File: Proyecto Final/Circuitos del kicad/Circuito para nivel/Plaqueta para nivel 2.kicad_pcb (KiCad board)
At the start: 2 copper layers, 60 x 44 mm, 20 parts, among them J1 Conn_01x05, J2 Conn_01x03, Q1 BC557, Q2 BC557, Q3 BC557, Q4 BC557, U1 ULN2003A

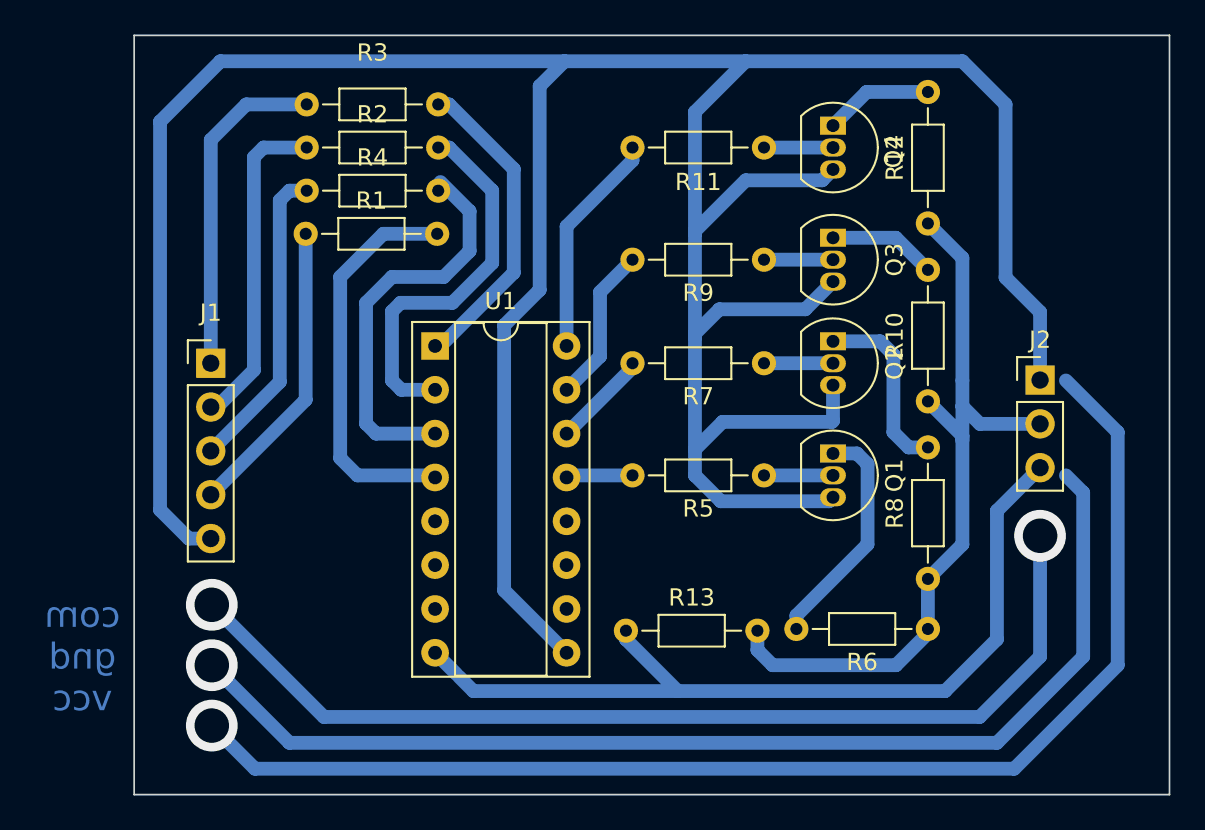
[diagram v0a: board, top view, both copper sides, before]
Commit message: Placas bien subidas
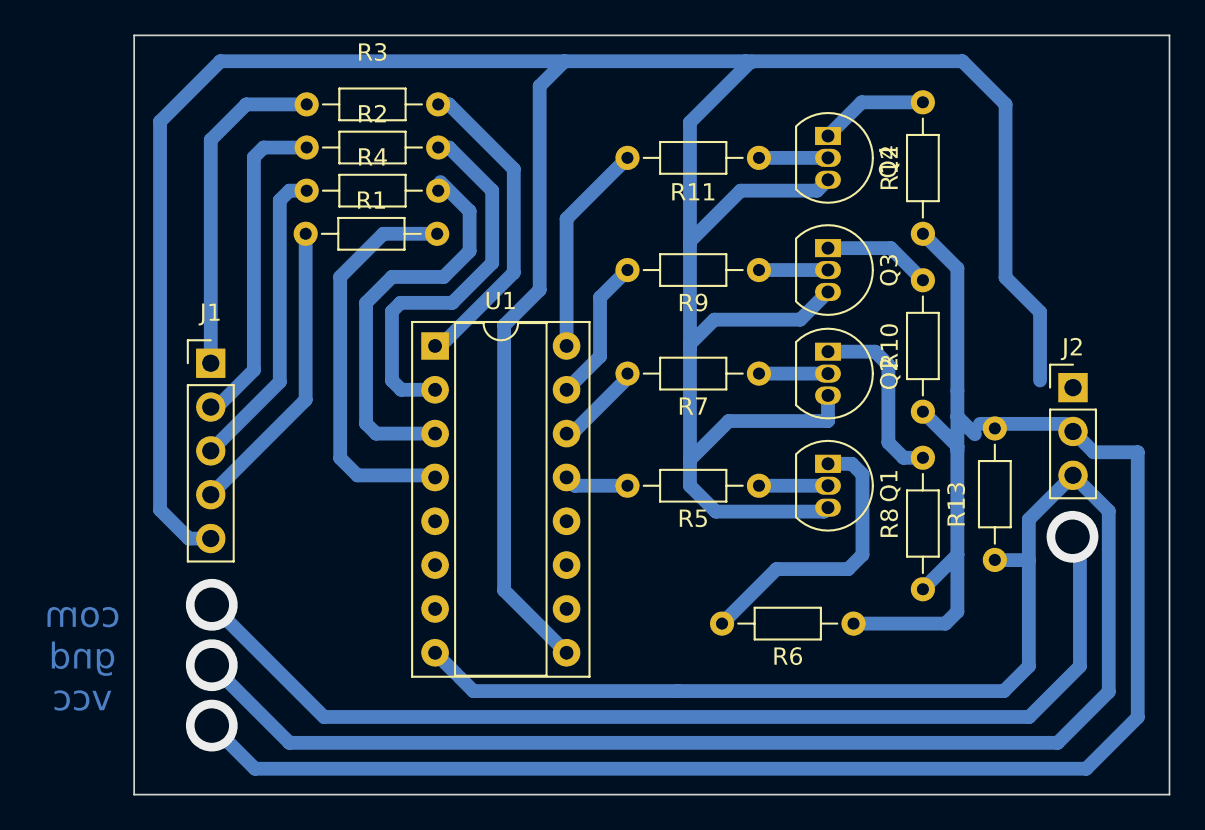
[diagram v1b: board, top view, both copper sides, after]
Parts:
- moved R13 21.8 mm to (158.9, 116.9), turned to 90 degrees
- moved R6 4.32 mm to (150.7, 120.6)
- moved J2 1.96 mm to (163.4, 106.9)
- moved R10 0.67 mm to (154.7, 108.3)
- moved Q1 0.67 mm to (149.2, 111.3)
- moved Q2 0.67 mm to (149.2, 104.8)
- moved Q3 0.67 mm to (149.2, 98.8)
- moved Q4 0.67 mm to (149.2, 92.3)
- moved R11 0.67 mm to (145.2, 93.6)
- moved R12 0.67 mm to (154.7, 98.0)
- moved R5 0.67 mm to (145.2, 112.6)
- moved R7 0.67 mm to (145.2, 106.1)
- moved R8 0.67 mm to (154.7, 118.6)
- moved R9 0.67 mm to (145.2, 100.1)
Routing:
- net GND: track 96.0 -> 297.9 mm
- net (no net): track 198.3 -> 0.00 mm
- net Net-(Q1-Pad1): track 13.5 -> 16.7 mm
- net Net-(R9-Pad2): track 9.12 -> 8.40 mm
- net Net-(R11-Pad2): track 13.1 -> 12.4 mm
- net +5V: track 195.5 -> 196.1 mm
- net Net-(R7-Pad2): track 5.66 -> 5.12 mm

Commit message: jhjkhn
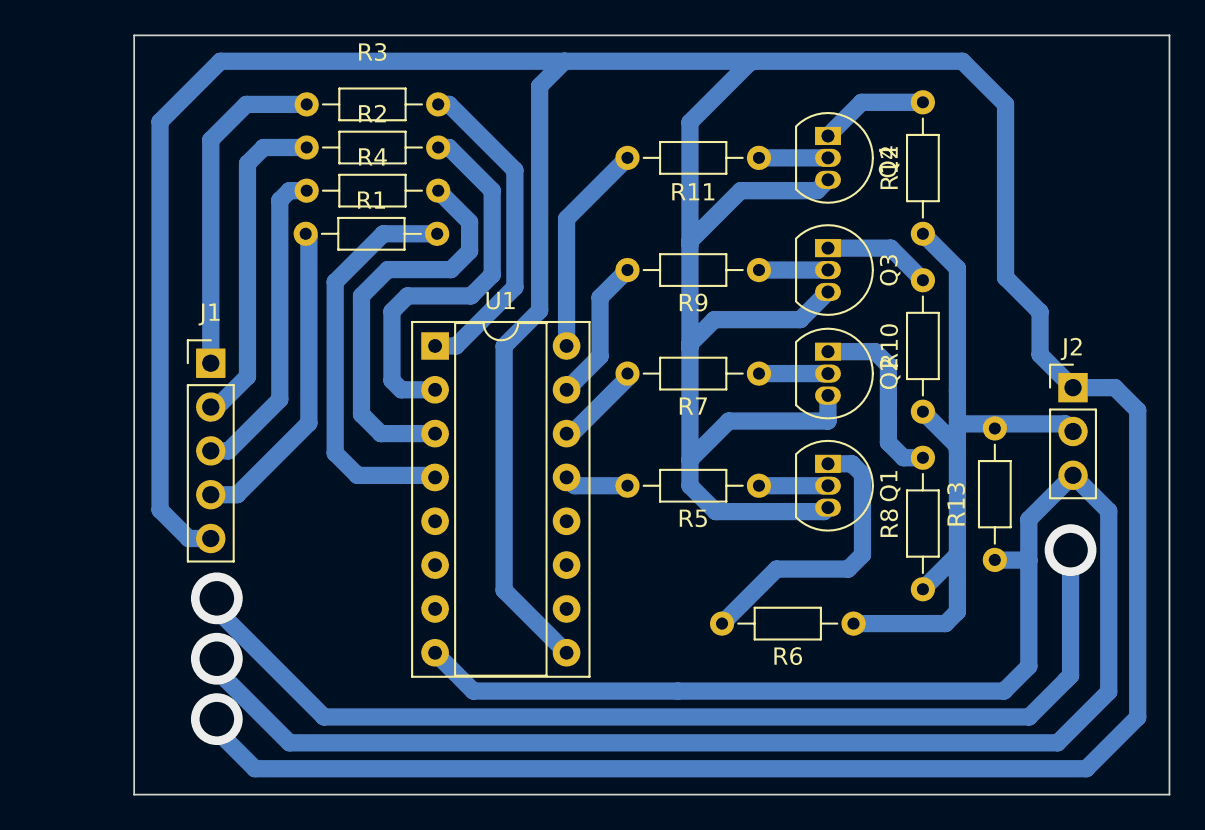
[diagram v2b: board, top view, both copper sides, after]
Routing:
- net +5V: track 196.1 -> 275.3 mm, vias 0 -> 1
- net GND: track 297.9 -> 221.1 mm, vias 0 -> 1
- net Net-(J1-Pad4): track 17.4 -> 18.4 mm
- net Net-(J1-Pad3): track 18.0 -> 18.6 mm
- net Net-(R3-Pad2): track 18.3 -> 18.8 mm
- net (no net): vias 4 -> 2
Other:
- board text removed: "com gnd vcc"

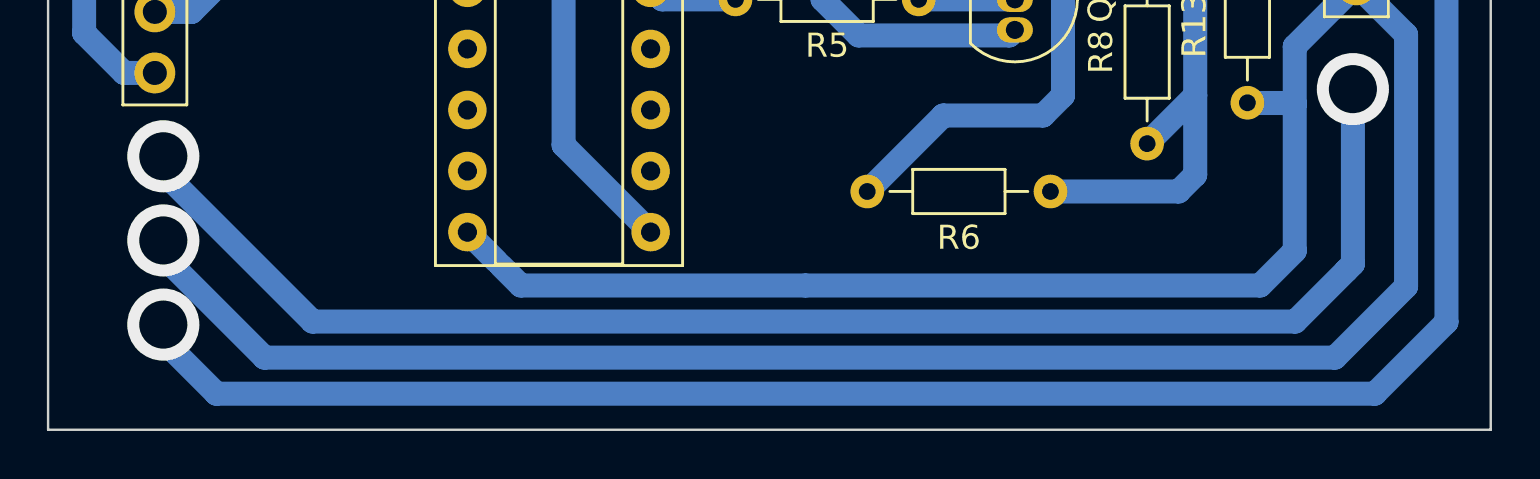
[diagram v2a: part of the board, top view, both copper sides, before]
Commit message: |a
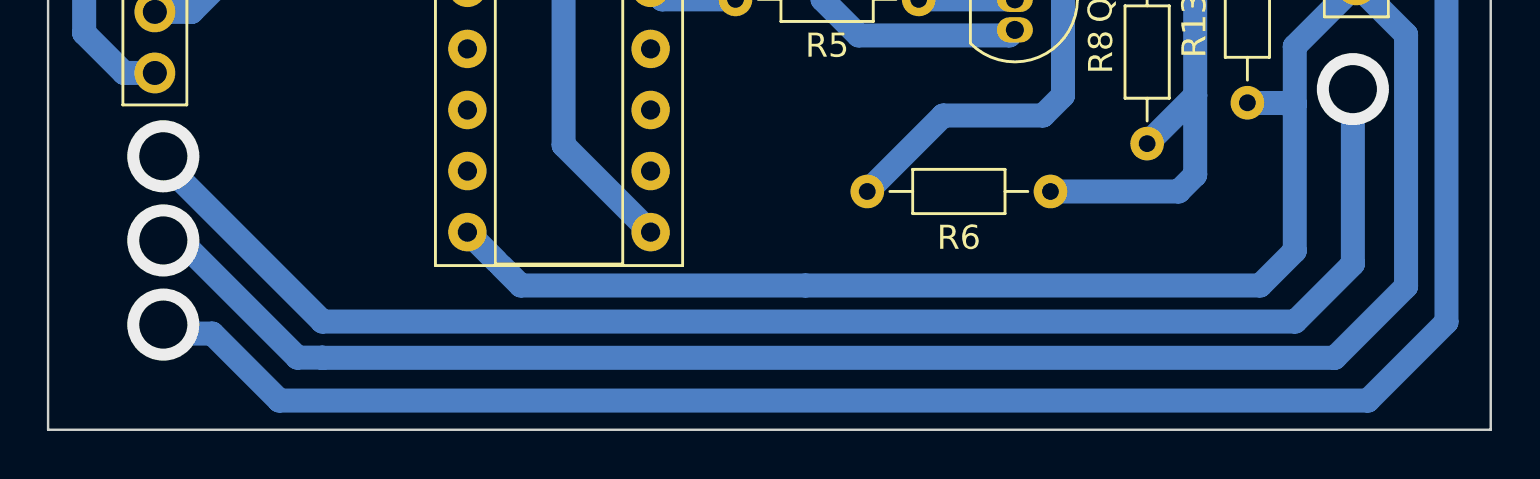
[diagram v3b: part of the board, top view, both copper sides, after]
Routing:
- net GND: track 221.1 -> 220.9 mm, vias 1 -> 3
- net (no net): vias 2 -> 0
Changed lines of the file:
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@@
   )
   (gr_rect (start 169 130.5) (end 109 86.5) (layer "Edge.Cuts") (width 0.1) (fill none))
-  (via (at 113.792 122.626) (size 3) (drill 2) (layers "F.Cu" "B.Cu") (free) (net 0))
-  (via (at 113.792 119.126) (size 3) (drill 2) (layers "F.Cu" "B.Cu") (free) (net 0))
   (segment (start 151.21 111.942345) (end 151.21 116.6) (width 1) (layer "B.Cu") (net 1))
   (segment (start 150.38 117.43) (end 146.23 117.43) (width 1) (layer "B.Cu") (net 1))
@@
   (segment (start 114 88) (end 133.94 88) (width 1) (layer "B.Cu") (net 3))
   (segment (start 130.44 118.66) (end 134.06 122.28) (width 1) (layer "B.Cu") (net 3))
-  (segment (start 164.18 129) (end 116 129) (width 1) (layer "B.Cu") (net 3))
+  (segment (start 167.16 108.232) (end 167.16 126.02) (width 1) (layer "B.Cu") (net 3))
   (segment (start 144.15 95.5) (end 148.58 95.5) (width 1) (layer "B.Cu") (net 3))
   (segment (start 159.5 90.5) (end 159.5 100.535) (width 1) (layer "B.Cu") (net 3))
   (segment (start 142.71 114.1) (end 141.21 112.6) (width 1) (layer "B.Cu") (net 3))
+  (segment (start 163.41 106.915) (end 165.843 106.915) (width 1) (layer "B.Cu") (net 3))
   (segment (start 112.16 115.66) (end 110.5 114) (width 1) (layer "B.Cu") (net 3))
   (segment (start 141.21 104.6) (end 141.21 98.44) (width 1) (layer "B.Cu") (net 3))
+  (segment (start 115.832 126.5) (end 113.5 126.5) (width 1) (layer "B.Cu") (net 3))
+  (segment (start 118.618 129.286) (end 115.832 126.5) (width 1) (layer "B.Cu") (net 3))
   (segment (start 147.605 102.975) (end 149.21 101.37) (width 1) (layer "B.Cu") (net 3))
   (segment (start 141.21 104.39) (end 142.625 102.975) (width 1) (layer "B.Cu") (net 3))
@@
   (segment (start 113.44 115.66) (end 112.16 115.66) (width 1) (layer "B.Cu") (net 3))
   (segment (start 132.5 102.45) (end 130.44 104.51) (width 1) (layer "B.Cu") (net 3))
-  (segment (start 165.843 106.915) (end 167.16 108.232) (width 1) (layer "B.Cu") (net 3))
   (segment (start 149.21 108.84) (end 149.21 107.37) (width 1) (layer "B.Cu") (net 3))
+  (segment (start 163.894 129.286) (end 118.618 129.286) (width 1) (layer "B.Cu") (net 3))
   (segment (start 110.5 91.5) (end 114 88) (width 1) (layer "B.Cu") (net 3))
   (segment (start 144.87 88.03) (end 144.72 88.03) (width 1) (layer "B.Cu") (net 3))
@@
   (segment (start 161.5 102.535) (end 161.5 105.005) (width 1) (layer "B.Cu") (net 3))
   (segment (start 157 88) (end 159.5 90.5) (width 1) (layer "B.Cu") (net 3))
+  (segment (start 165.843 106.915) (end 167.16 108.232) (width 1) (layer "B.Cu") (net 3))
   (segment (start 132.5 89.44) (end 132.5 102.45) (width 1) (layer "B.Cu") (net 3))
   (segment (start 142.625 102.975) (end 147.605 102.975) (width 1) (layer "B.Cu") (net 3))
+  (segment (start 167.16 126.02) (end 163.894 129.286) (width 1) (layer "B.Cu") (net 3))
   (segment (start 149.21 113.87) (end 148.98 114.1) (width 1) (layer "B.Cu") (net 3))
   (segment (start 148.98 114.1) (end 142.71 114.1) (width 1) (layer "B.Cu") (net 3))
@@
   (segment (start 141.21 111.1) (end 143.46 108.85) (width 1) (layer "B.Cu") (net 3))
   (segment (start 141.21 98.44) (end 144.15 95.5) (width 1) (layer "B.Cu") (net 3))
-  (segment (start 167.16 108.232) (end 167.16 126.02) (width 1) (layer "B.Cu") (net 3))
-  (segment (start 116 129) (end 113.5 126.5) (width 1) (layer "B.Cu") (net 3))
-  (segment (start 163.41 106.915) (end 165.843 106.915) (width 1) (layer "B.Cu") (net 3))
   (segment (start 141.21 111.1) (end 141.21 104.39) (width 1) (layer "B.Cu") (net 3))
   (segment (start 161.5 105.005) (end 163.41 106.915) (width 1) (layer "B.Cu") (net 3))
   (segment (start 159.5 100.535) (end 161.5 102.535) (width 1) (layer "B.Cu") (net 3))
   (segment (start 149.2 108.85) (end 149.21 108.84) (width 1) (layer "B.Cu") (net 3))
-  (segment (start 167.16 126.02) (end 164.18 129) (width 1) (layer "B.Cu") (net 3))
   (segment (start 133.94 88) (end 132.5 89.44) (width 1) (layer "B.Cu") (net 3))
   (segment (start 152.71 110.1) (end 153.59 110.98) (width 1) (layer "B.Cu") (net 4))
@@
   (segment (start 119.126 98.186) (end 118.94 98) (width 1) (layer "B.Cu") (net 27))
   (via (at 163.268053 116.332672) (size 3) (drill 2) (layers "F.Cu" "B.Cu") (free) (net 28))
+  (via (at 113.792 122.626) (size 3) (drill 2) (layers "F.Cu" "B.Cu") (free) (net 28))
+  (via (at 113.792 119.126) (size 3) (drill 2) (layers "F.Cu" "B.Cu") (free) (net 28))
   (segment (start 154.71 108.31) (end 156.71 110.31) (width 1) (layer "B.Cu") (net 28))
+  (segment (start 120.412 127.508) (end 162.512 127.508) (width 1) (layer "B.Cu") (net 28))
   (segment (start 154.71 108.31) (end 154.92 108.31) (width 1) (layer "B.Cu") (net 28))
   (segment (start 156.71 110.31) (end 156.71 116.6) (width 1) (layer "B.Cu") (net 28))
-  (segment (start 163.268053 123.601947) (end 162.993 123.877) (width 1) (layer "B.Cu") (net 28))
   (segment (start 158.78 116.91) (end 160.71 116.91) (width 1) (layer "B.Cu") (net 28))
-  (segment (start 162.52 127.5) (end 165.48 124.54) (width 1) (layer "B.Cu") (net 28))
+  (segment (start 119.372 127.5) (end 120.404 127.5) (width 1) (layer "B.Cu") (net 28))
   (segment (start 159.41 124.5) (end 140.5 124.5) (width 1) (layer "B.Cu") (net 28))
   (segment (start 156.718 108.966) (end 156.767 109.015) (width 1) (layer "B.Cu") (net 28))
-  (segment (start 162.993 123.877) (end 160.87 126) (width 1) (layer "B.Cu") (net 28))
-  (segment (start 118 127.5) (end 162.52 127.5) (width 1) (layer "B.Cu") (net 28))
   (segment (start 160.85 123.06) (end 159.41 124.5) (width 1) (layer "B.Cu") (net 28))
   (segment (start 128.66 124.5) (end 127.839511 123.679511) (width 1) (layer "B.Cu") (net 28))
-  (segment (start 120 126) (end 113.5 119.5) (width 1) (layer "B.Cu") (net 28))
   (segment (start 160.81 116.9) (end 160.85 116.94) (width 1) (layer "B.Cu") (net 28))
   (segment (start 163.41 111.995) (end 160.85 114.555) (width 1) (layer "B.Cu") (net 28))
-  (segment (start 113.5 123) (end 118 127.5) (width 1) (layer "B.Cu") (net 28))
+  (segment (start 113.792 119.38) (end 113.792 119.126) (width 1) (layer "B.Cu") (net 28))
   (segment (start 150.69 120.59) (end 156.02 120.59) (width 1) (layer "B.Cu") (net 28))
+  (segment (start 160.87 126) (end 120.412 126) (width 1) (layer "B.Cu") (net 28))
   (segment (start 163.268053 116.332672) (end 163.268053 123.601947) (width 1) (layer "B.Cu") (net 28))
   (segment (start 156.71 116.6) (end 154.71 118.6) (width 1) (layer "B.Cu") (net 28))
+  (segment (start 165.48 124.54) (end 165.48 114.065) (width 1) (layer "B.Cu") (net 28))
   (segment (start 156.02 120.59) (end 156.71 119.9) (width 1) (layer "B.Cu") (net 28))
   (segment (start 127.66 123.5) (end 126.44 122.28) (width 1) (layer "B.Cu") (net 28))
   (segment (start 156.767 109.015) (end 162.97 109.015) (width 1) (layer "B.Cu") (net 28))
+  (segment (start 113.792 122.626) (end 114.498 122.626) (width 1) (layer "B.Cu") (net 28))
+  (segment (start 162.512 127.508) (end 165.48 124.54) (width 1) (layer "B.Cu") (net 28))
   (segment (start 162.97 109.015) (end 163.41 109.455) (width 1) (layer "B.Cu") (net 28))
   (segment (start 156.71 119.9) (end 156.71 116.6) (width 1) (layer "B.Cu") (net 28))
   (segment (start 160.85 116.94) (end 160.85 123.06) (width 1) (layer "B.Cu") (net 28))
-  (segment (start 165.48 114.065) (end 163.41 111.995) (width 1) (layer "B.Cu") (net 28))
+  (segment (start 120.412 126) (end 113.792 119.38) (width 1) (layer "B.Cu") (net 28))
   (segment (start 154.71 98) (end 156.71 100) (width 1) (layer "B.Cu") (net 28))
   (segment (start 160.85 114.555) (end 160.85 116.94) (width 1) (layer "B.Cu") (net 28))
   (segment (start 156.71 100) (end 156.71 107.1) (width 1) (layer "B.Cu") (net 28))
+  (segment (start 120.404 127.5) (end 120.412 127.508) (width 1) (layer "B.Cu") (net 28))
+  (segment (start 165.48 114.065) (end 163.41 111.995) (width 1) (layer "B.Cu") (net 28))
   (segment (start 156.71 108.6) (end 156.71 110.6) (width 1) (layer "B.Cu") (net 28))
-  (segment (start 165.48 124.54) (end 165.48 114.065) (width 1) (layer "B.Cu") (net 28))
+  (segment (start 114.498 122.626) (end 119.372 127.5) (width 1) (layer "B.Cu") (net 28))
   (segment (start 140.5 124.5) (end 128.66 124.5) (width 1) (layer "B.Cu") (net 28))
-  (segment (start 160.87 126) (end 120 126) (width 1) (layer "B.Cu") (net 28))
+  (segment (start 163.268053 123.601947) (end 160.87 126) (width 1) (layer "B.Cu") (net 28))
   (segment (start 156.71 107.1) (end 156.71 108.6) (width 1) (layer "B.Cu") (net 28))
 )
